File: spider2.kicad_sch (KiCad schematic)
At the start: 104 parts, among them J1 NRJ6HH, J10 PJ-320A, J11 PJ359, J12 PJ359, J13 PJ359, J14 PJ359, J15 PJ359, J16 PJ359, J17 A, J19 PJ359, J2 NRJ6HH, J20 PJ359, J3 PJ359, J4 PJ359, J5 PJ359, J6 PJ-320A, J7 PJ359, J8 PJ359, J9 PJ359, P1 USB4085, Q1 AOI4286, Q2 BC547, Q3 BC547, SW4 200MDP3T1B1M6QE, U2 AP63203WU, U4 NE5532, U7 PAM8406D

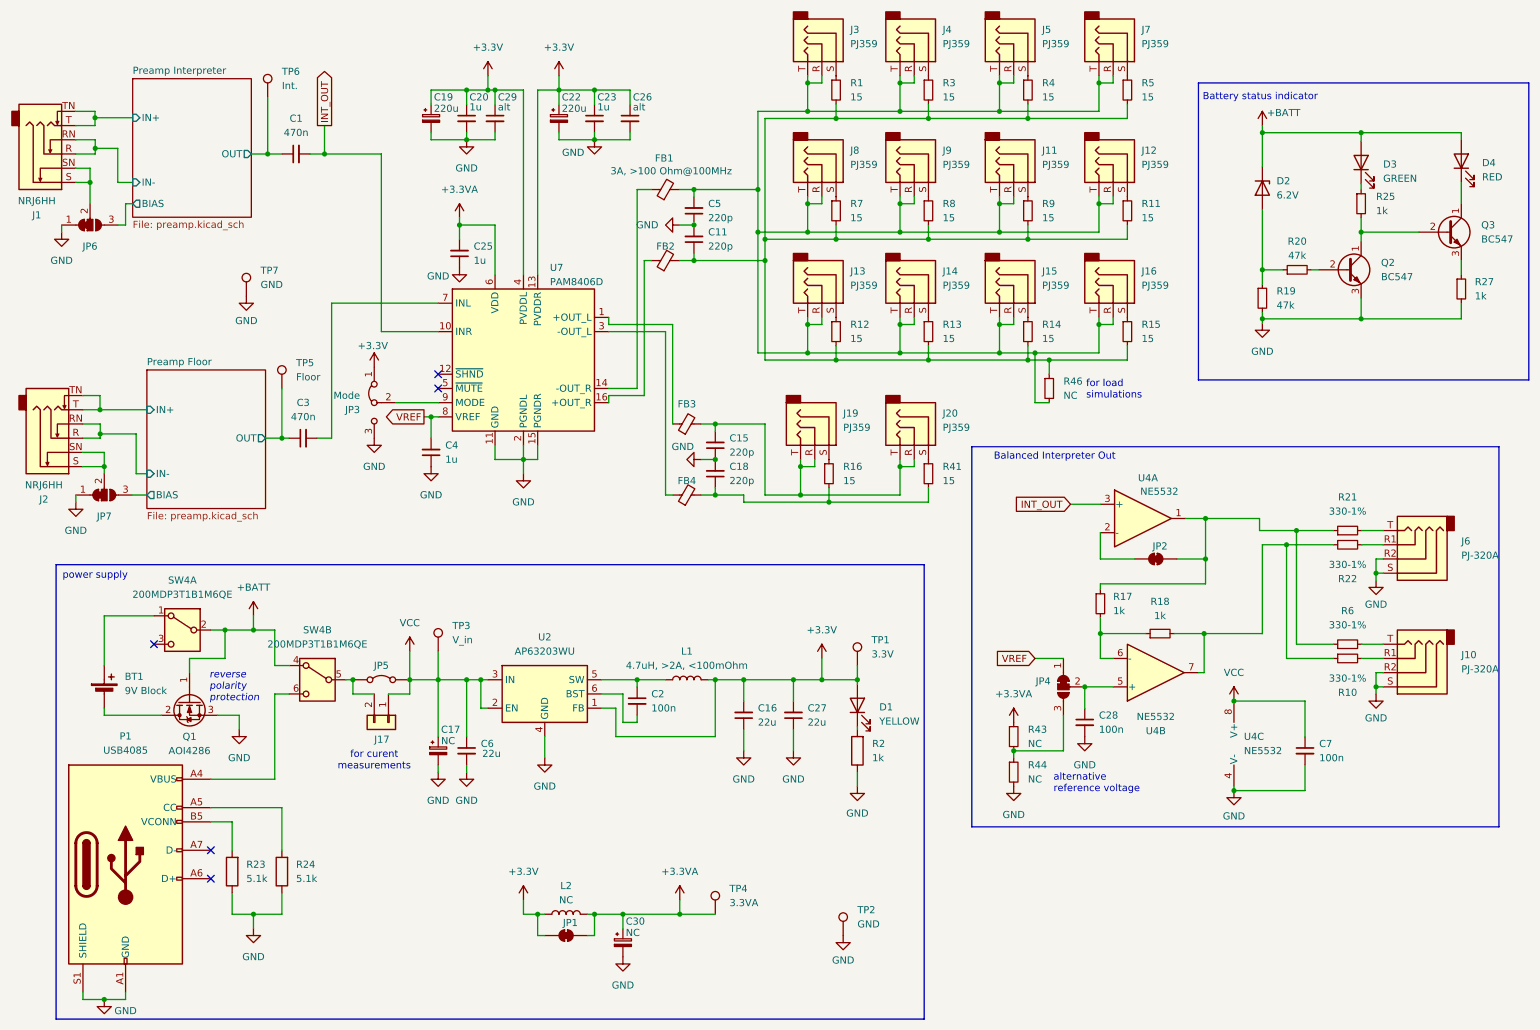
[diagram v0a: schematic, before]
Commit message: implement review feedback
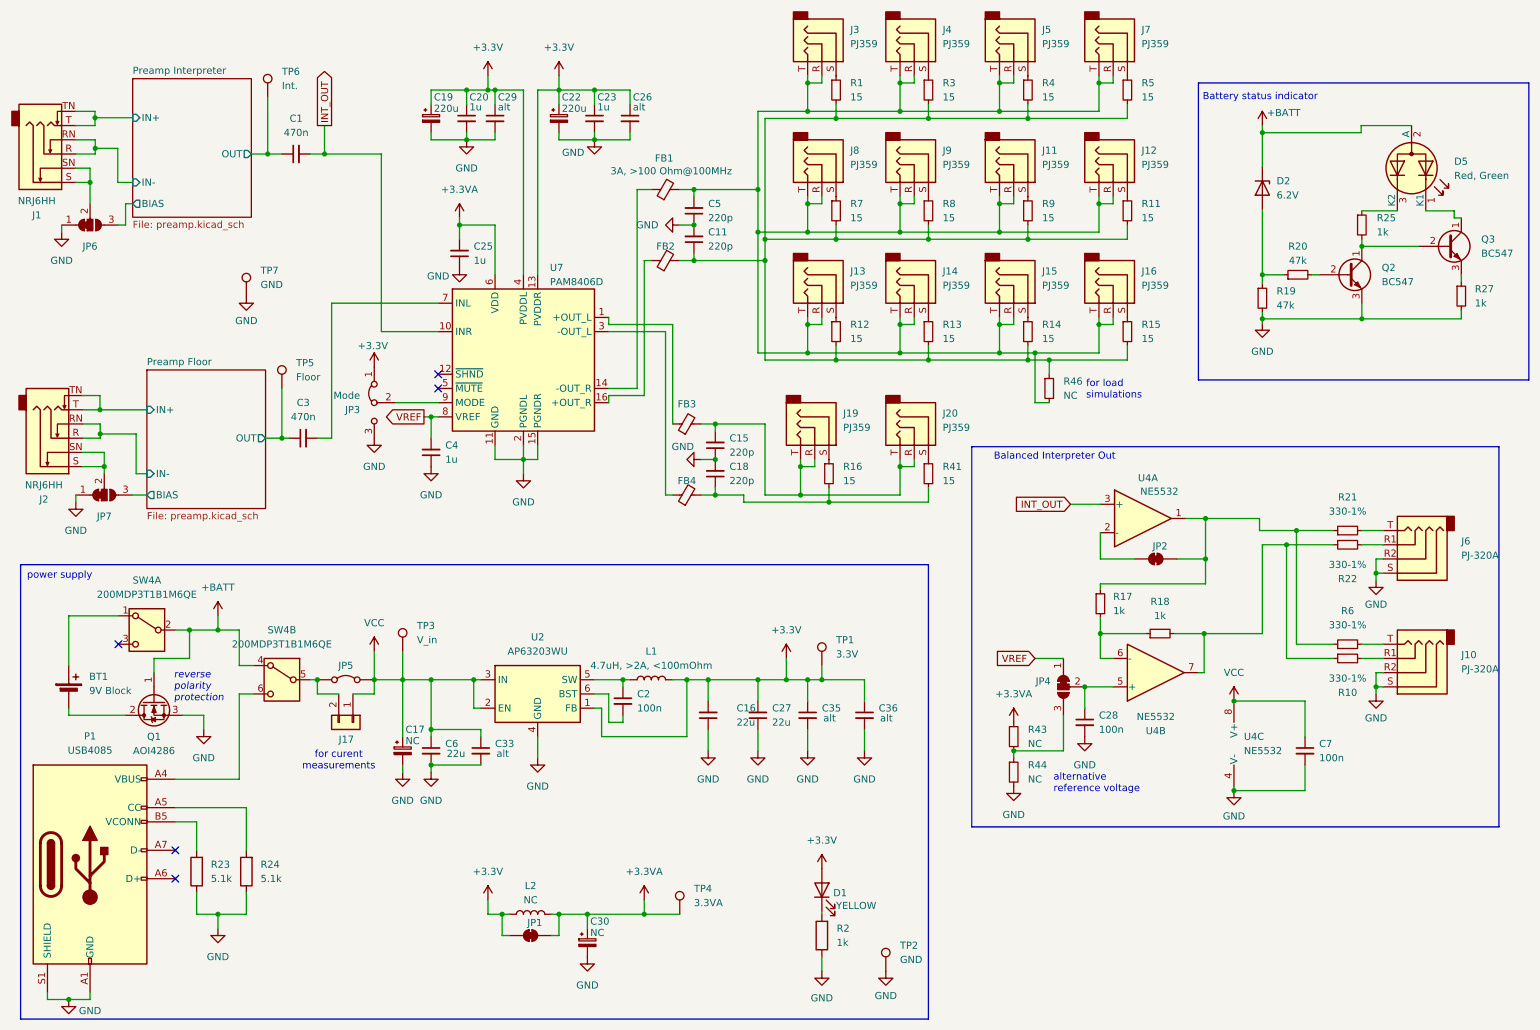
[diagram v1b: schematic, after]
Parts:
- removed D3: GREEN, LED_THT:LED_D3.0mm_FlatTop, symbol Device:LED
- removed D4: RED, LED_THT:LED_D3.0mm_FlatTop, symbol Device:LED
- added C33, C35, C36: alt, Capacitor_SMD:C_1210_3225Metric_Pad1.33x2.70mm_HandSolder, symbol Device:C_Small
- added D5: Red, Green, LED_THT:LED_D5.0mm-3, symbol Device:LED_Dual_KAK
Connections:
- net +3.3V: now also C35.1, C36.1
- net +BATT: now also D5.2 (A)
- net GND: now also C33.2, C35.2, C36.2
- net VCC: now also C33.1
- net at R25.1: now also D5.3 (K2)
- net at Q3.1 (C): now also D5.1 (K1)
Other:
- moved on the sheet: BT1, C16, C17, C2, C27, C30, C6, J17, JP1, JP5, L1, L2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
